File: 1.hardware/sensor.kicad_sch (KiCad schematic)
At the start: 13 parts, among them U10 Hall_Analog_Joystick, U2 LM75B, U9 Hall_Analog_Joystick

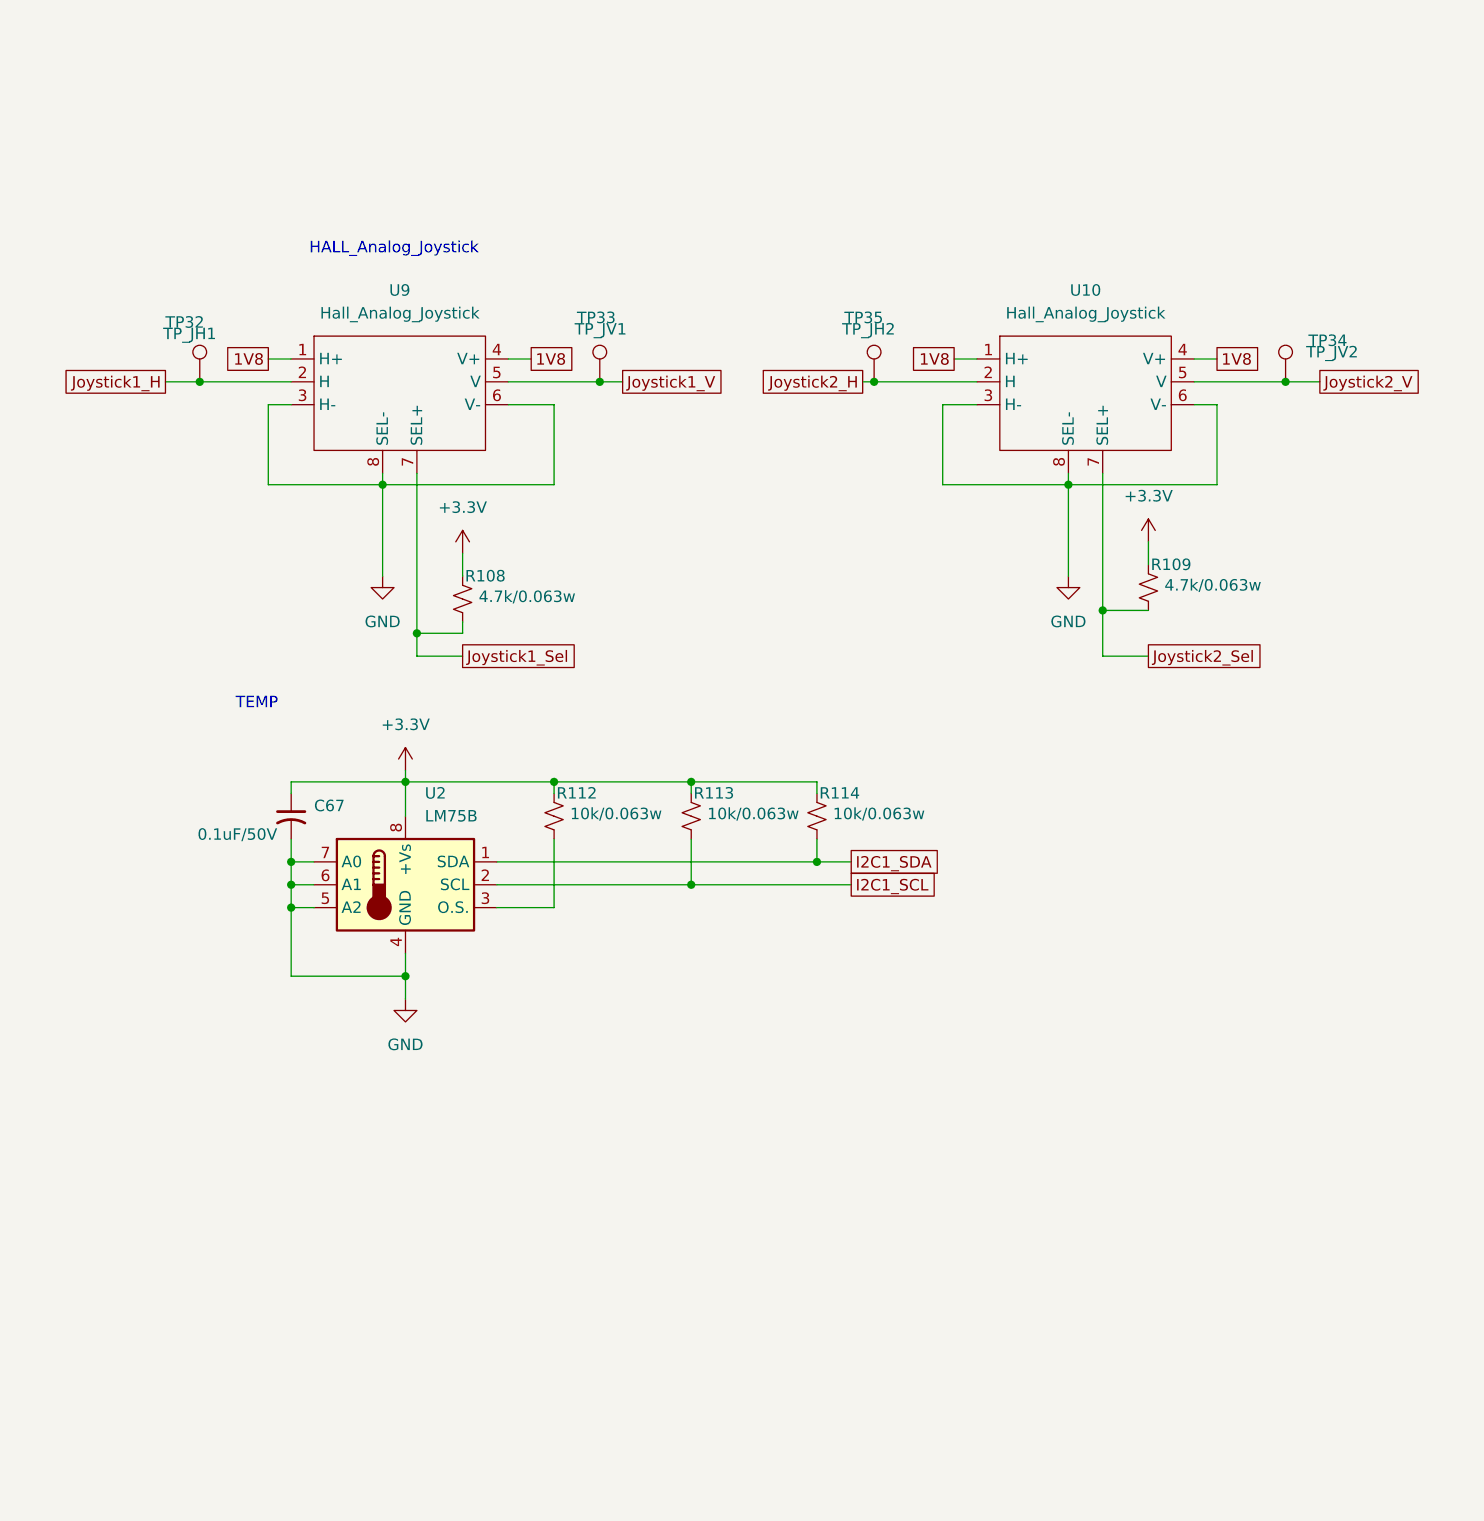
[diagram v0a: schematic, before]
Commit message: 중간 저장
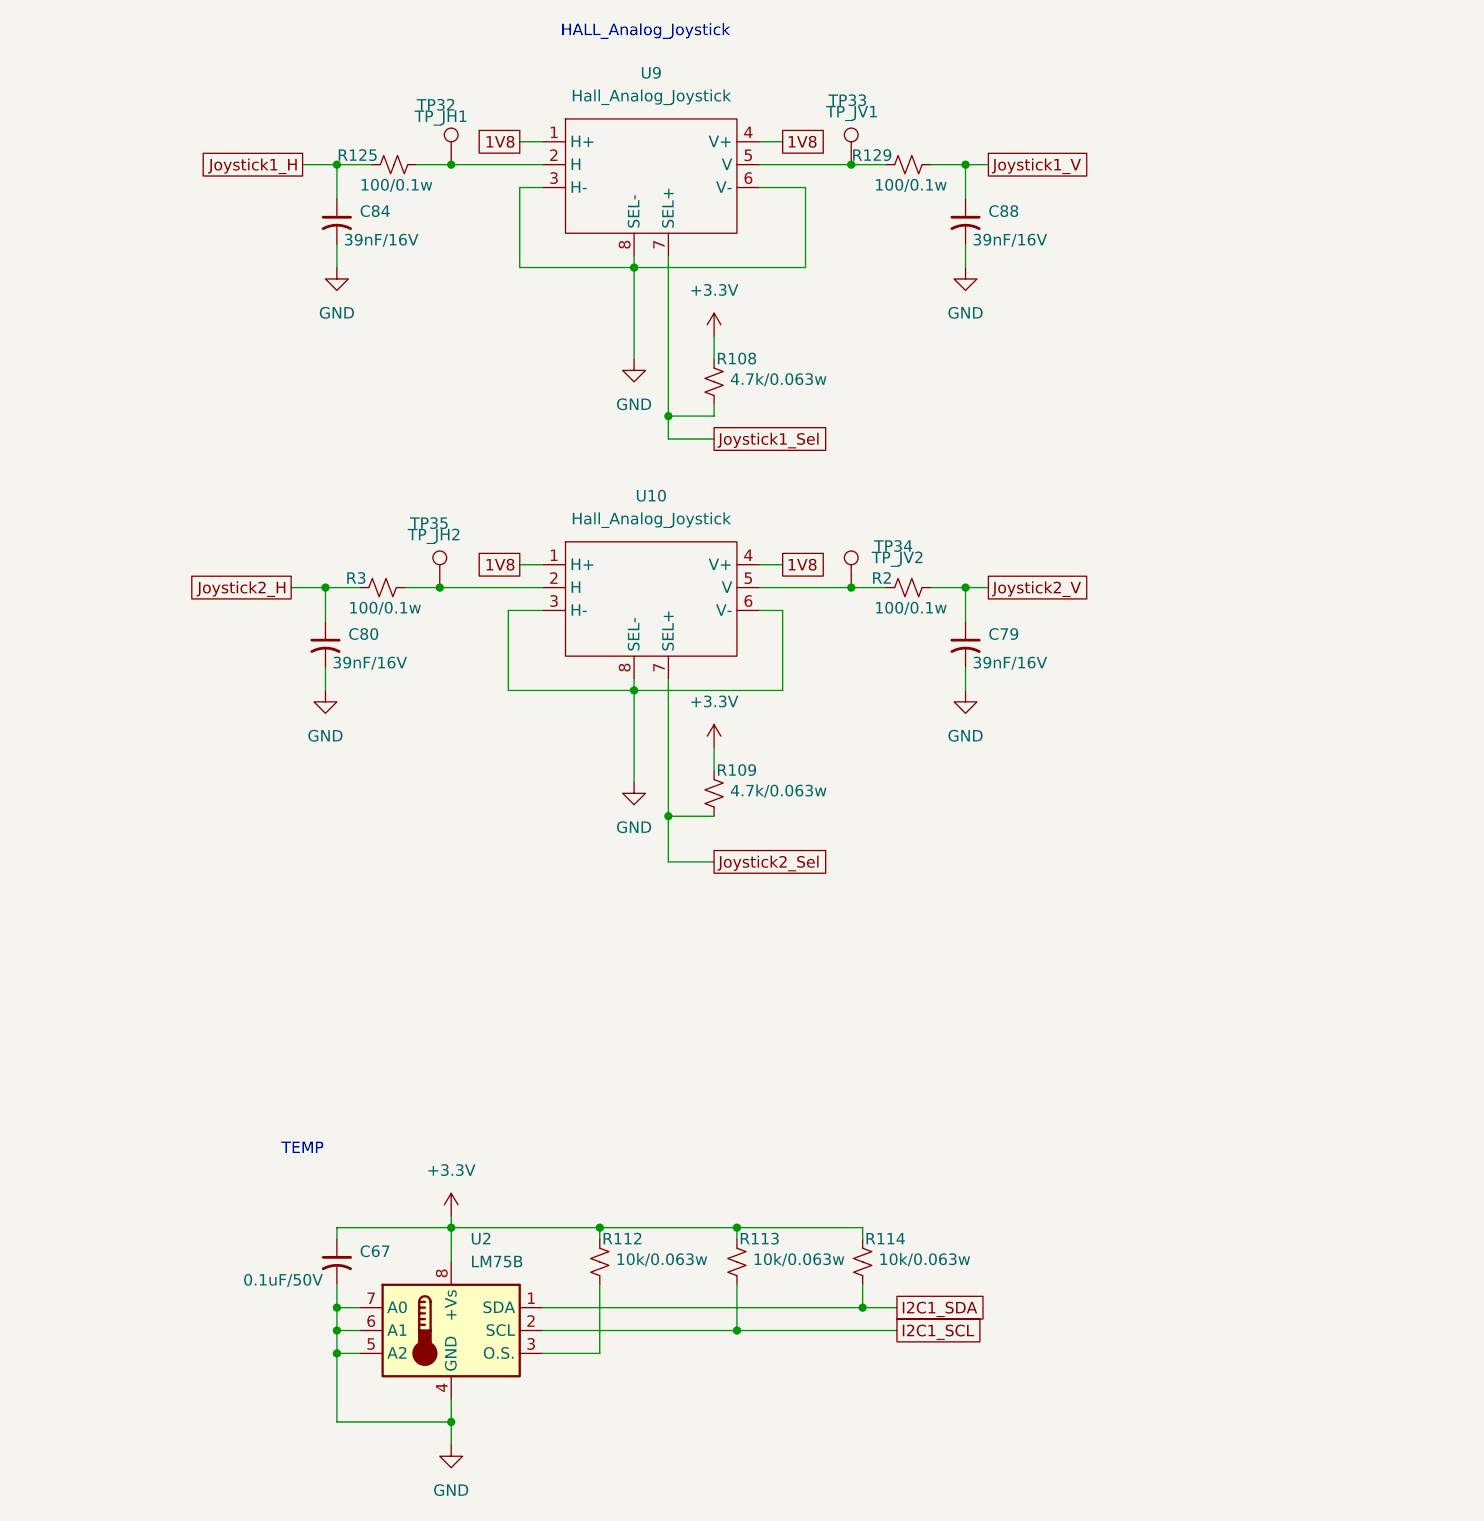
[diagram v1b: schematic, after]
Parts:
- added C79, C80, C84, C88: 39nF/16V, symbol Device:C_Small_US
- added R125, R129, R2, R3: 100/0.1w, Resistor_SMD:R_0402_1005Metric, symbol Device:R_Small_US
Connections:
- net GND: now also C79.2, C80.2, C84.2, C88.2
- net Joystick1_H: now also C84.1, R125.1; no longer TP32.1, U9.2 (H)
- net Joystick1_V: now also C88.1, R129.2; no longer TP33.1, U9.5 (V)
- net Joystick2_H: now also C80.1, R3.1; no longer TP35.1, U10.2 (H)
- net Joystick2_V: now also C79.1, R2.2; no longer TP34.1, U10.5 (V)
- new net: R3.2, TP35.1, U10.2 (H)
- new net: R125.2, TP32.1, U9.2 (H)
- new net: R2.1, TP34.1, U10.5 (V)
- new net: R129.1, TP33.1, U9.5 (V)
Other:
- moved on the sheet: C67, R108, R109, R112, R113, R114, TP32, TP33, TP34, TP35, U10, U2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

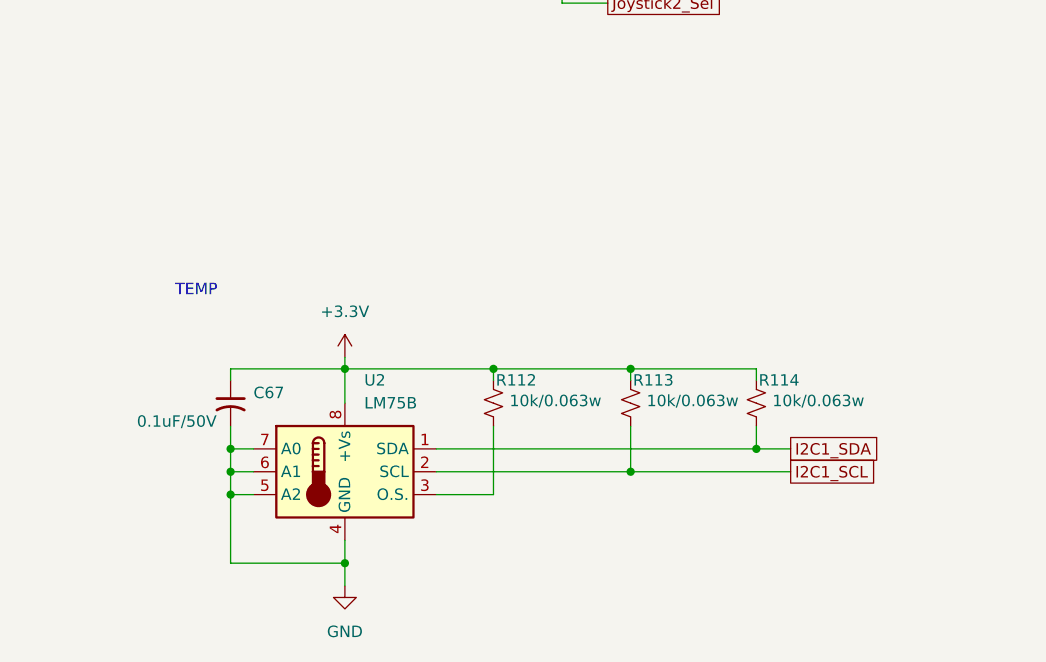
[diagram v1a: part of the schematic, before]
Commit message: 핀 배치 완료
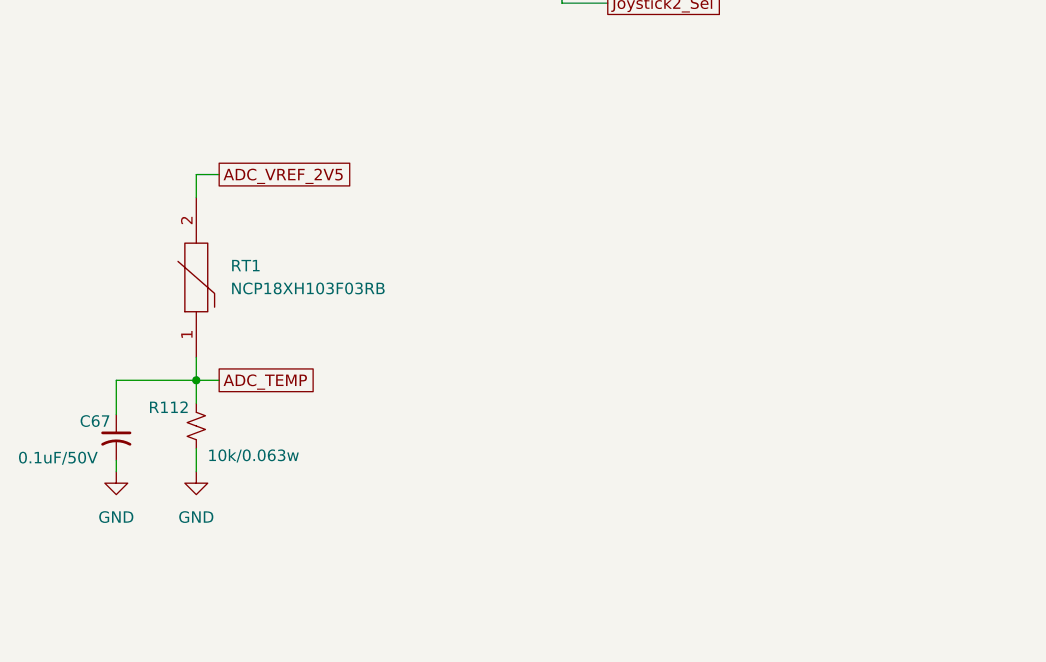
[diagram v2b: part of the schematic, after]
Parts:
- removed R113, R114: 10k/0.063w, Resistor_SMD:R_0402_1005Metric, symbol Device:R_Small_US
- removed U2: LM75B, symbol Sensor_Temperature:LM75B
- added RT1: NCP18XH103F03RB, THRMC1608X95N, symbol SamacSys_Parts:NCP18XH103F03RB
- R112: footprint Resistor_SMD:R_0402_1005Metric -> (none)
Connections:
- net +3.3V: no longer C67.1, R112.1
- net GND: now also R112.1
- net ADC_TEMP: now reaches R112.2
- net ADC_TEMP: now also C67.1, RT1.1
- new net ADC_VREF_2V5: RT1.2
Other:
- note removed: "TEMP"
